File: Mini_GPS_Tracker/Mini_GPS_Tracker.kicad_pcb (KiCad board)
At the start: 2 copper layers, 42 parts, among them J1 USB_C_Receptacle, J2 Screw_Terminal_01x02, J3 901-10512-1, J4 Conn_ARM_JTAG_SWD_10, SW1 SW_Push, U1 CH340E, U2 MS5611-01BA, U3 LD1117S33TR_SOT223, U4 MAX-8Q, U5 SGGP.12.4.A.02, U6 XBee_SMT, U7 LSM9DS1, Y1 Crystal

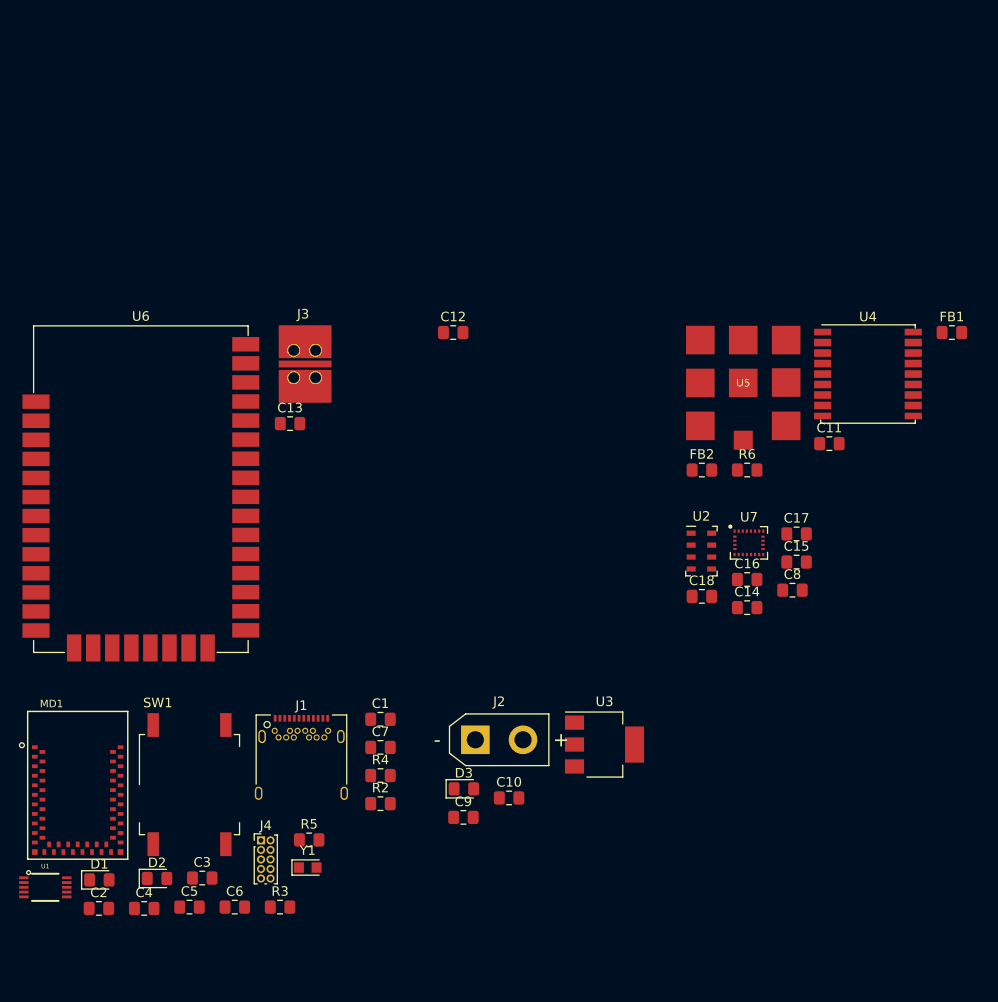
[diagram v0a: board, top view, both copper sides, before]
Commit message: schamatics finalized
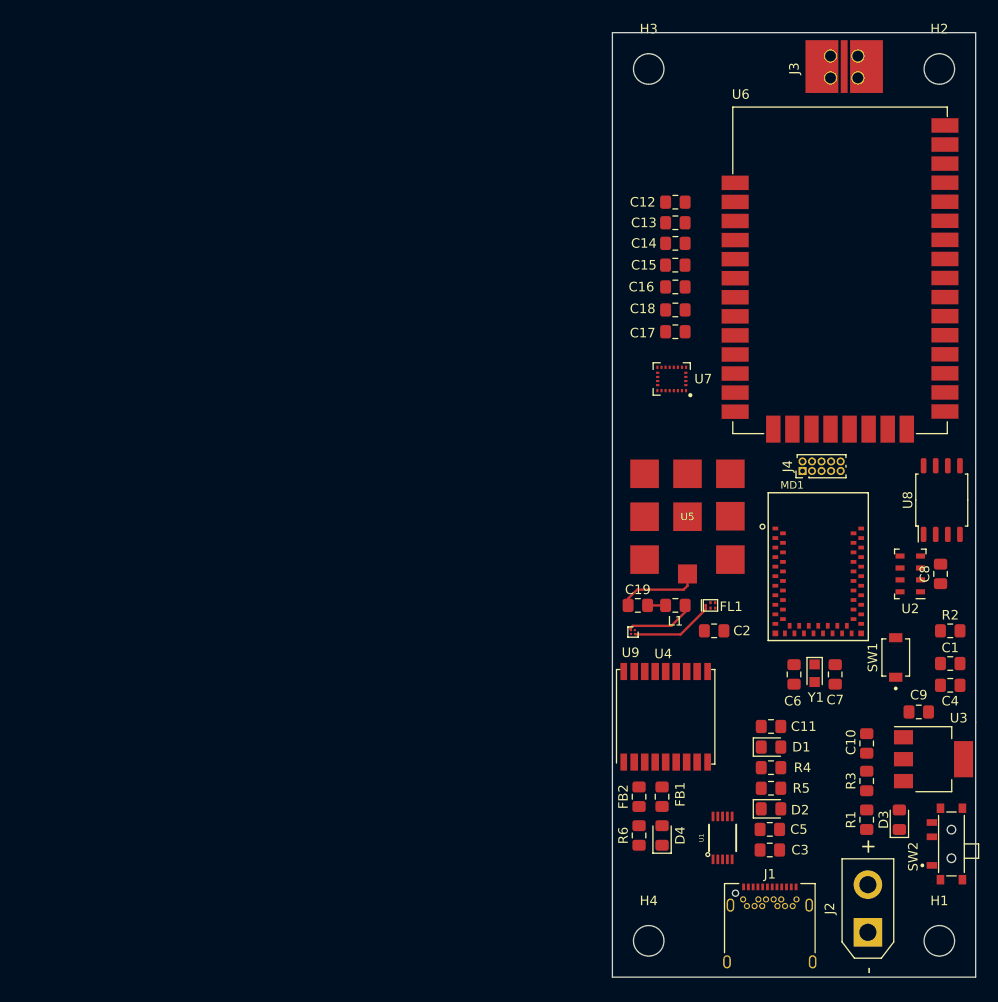
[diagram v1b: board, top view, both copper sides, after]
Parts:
- added C19: CAP, Capacitor_SMD:C_0805_2012Metric_Pad1.15x1.40mm_HandSolder, F.Cu at (150.0, 100.7)
- added D4: LED, LED_SMD:LED_0805_2012Metric_Pad1.15x1.40mm_HandSolder, F.Cu at (152.5, 124.8)
- added FL1: SAFFA1G58KA0F0A, Filter:Filter_1411-5_1.4x1.1mm, F.Cu at (157.6, 100.7)
- added H1: MountingHole_Pad, MountingHole:MountingHole_3.2mm_M3, F.Cu at (181.6, 135.9)
- added H2: MountingHole_Pad, MountingHole:MountingHole_3.2mm_M3, F.Cu at (181.6, 44.5)
- added H3: MountingHole_Pad, MountingHole:MountingHole_3.2mm_M3, F.Cu at (151.1, 44.5)
- added H4: MountingHole_Pad, MountingHole:MountingHole_3.2mm_M3, F.Cu at (151.1, 135.9)
- added L1: INDUCTOR, Inductor_SMD:L_0805_2012Metric_Pad1.15x1.40mm_HandSolder, F.Cu at (153.9, 100.7)
- added R1: 10k, Resistor_SMD:R_0805_2012Metric_Pad1.15x1.40mm_HandSolder, F.Cu at (174.0, 123.2)
- added SW2: MLL1200S, SW_MLL1200S, F.Cu at (182.9, 125.7)
- added U8: W25Q128JVS, Package_SO:SOIC-8_5.23x5.23mm_P1.27mm, F.Cu at (181.9, 89.7)
- added U9: MAX2686, Package_BGA:WLP-4_0.86x0.86mm_P0.4mm, F.Cu at (149.5, 103.5)
- C10: value 100nF -> 10uF
- R3: value 220K -> 3k
- SW1: footprint Button_Switch_SMD:SW_MEC_5GSH9 -> Sparkfun-Artemis:SW_TL1015AF160QG
- moved C4 87.7 mm to (182.8, 109.1), turned to 180 degrees
- moved MD1 81.0 mm to (168.9, 96.6)
- moved U6 76.8 mm to (171.2, 66.3)
- moved SW1 75.3 mm to (177.0, 106.2), turned to 90 degrees
- moved D1 71.8 mm to (164.0, 115.6)
- moved U1 71.2 mm to (158.9, 125.1), turned to 90 degrees
- moved C2 70.8 mm to (158.0, 103.4)
- moved J4 68.7 mm to (167.3, 86.6), turned to 90 degrees
- moved D2 64.8 mm to (164.0, 122.0)
- moved J3 64.6 mm to (171.6, 44.2), turned to 90 degrees
- moved C6 63.5 mm to (166.4, 108.0), turned to 270 degrees
- moved R3 62.9 mm to (174.0, 119.1), turned to 90 degrees
- moved R2 62.4 mm to (182.8, 103.4)
- moved C5 61.4 mm to (163.8, 124.2)
- moved C1 60.0 mm to (182.8, 106.8)
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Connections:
- C2 pad 1: BOOT -> Net-(C2-Pad1)
- C2 pad 2: RTS -> +3V3
- J1 pad S1: Net-(J1-PadS1) -> GND
- J2 pad 2: Net-(D3-Pad1) -> Net-(J2-Pad2)
- J4 pad 10: RESET_2 -> RESET
- J4 pad 8: GND -> Net-(J4-Pad8)
- MD1 pad 11: Net-(MD1-Pad11) -> cs_flash
- MD1 pad 13: Net-(MD1-Pad13) -> clk_flash
- MD1 pad 42: Net-(MD1-Pad42) -> v_measure
- MD1 pad 49: TXO -> TX0
- MD1 pad 50: nReset -> RESET
- MD1 pad 52: Net-(MD1-Pad52) -> 9_SDA
- MD1 pad 53: Net-(MD1-Pad53) -> 9_SCL
- MD1 pad 58: Net-(MD1-Pad58) -> gps_reset
- MD1 pad 6: Net-(MD1-Pad6) -> MISO_Flash
- MD1 pad 7: BOOT -> Net-(MD1-Pad7)
- MD1 pad 8: Net-(MD1-Pad8) -> MOSI_Flash
- R3 pad 1: BOOT -> v_measure
- R6 pad 2: Net-(R6-Pad2) -> Net-(D4-Pad2)
- U4 pad 11: Net-(R6-Pad2) -> Net-(FL1-Pad4)
- U4 pad 4: Net-(U4-Pad4) -> Net-(R6-Pad1)
- U4 pad 9: Net-(U4-Pad9) -> gps_reset
- U5 pad RF: Net-(R6-Pad1) -> Net-(C19-Pad1)
- U7 pad 2: /Sheet5E70BD5D/9_SCL -> 9_SCL
- U7 pad 4: /Sheet5E70BD5D/9_SDA -> 9_SDA
- U7 pad 5: /Sheet5E70BD5D/9_SDO_AG -> +3V3
- U7 pad 6: /Sheet5E70BD5D/9_SDO_M -> +3V3
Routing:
- net Net-(FL1-Pad1): track 0.00 -> 8.88 mm
- net Net-(C19-Pad1): track 0.00 -> 8.74 mm
- net Net-(L1-Pad1): track 0.00 -> 7.28 mm
- net Net-(C19-Pad2): track 0.00 -> 1.89 mm
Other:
- board outline added: 38.1 x 99.1 mm
